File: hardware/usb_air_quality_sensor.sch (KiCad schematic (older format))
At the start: 21 parts

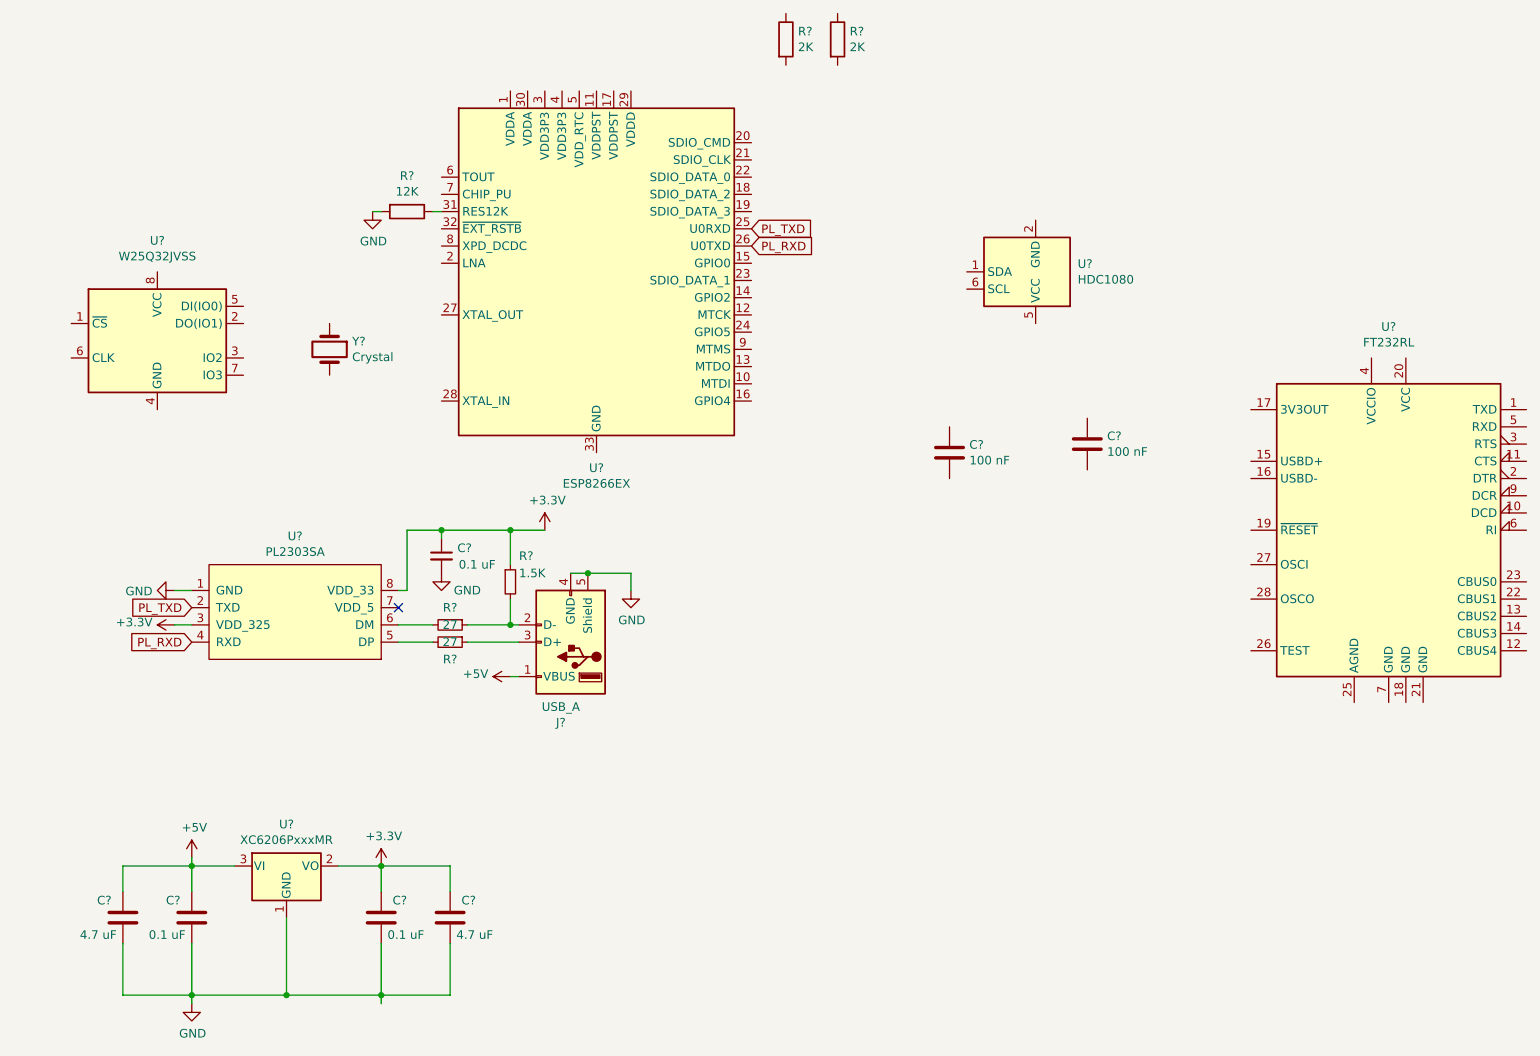
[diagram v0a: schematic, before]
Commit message: wip
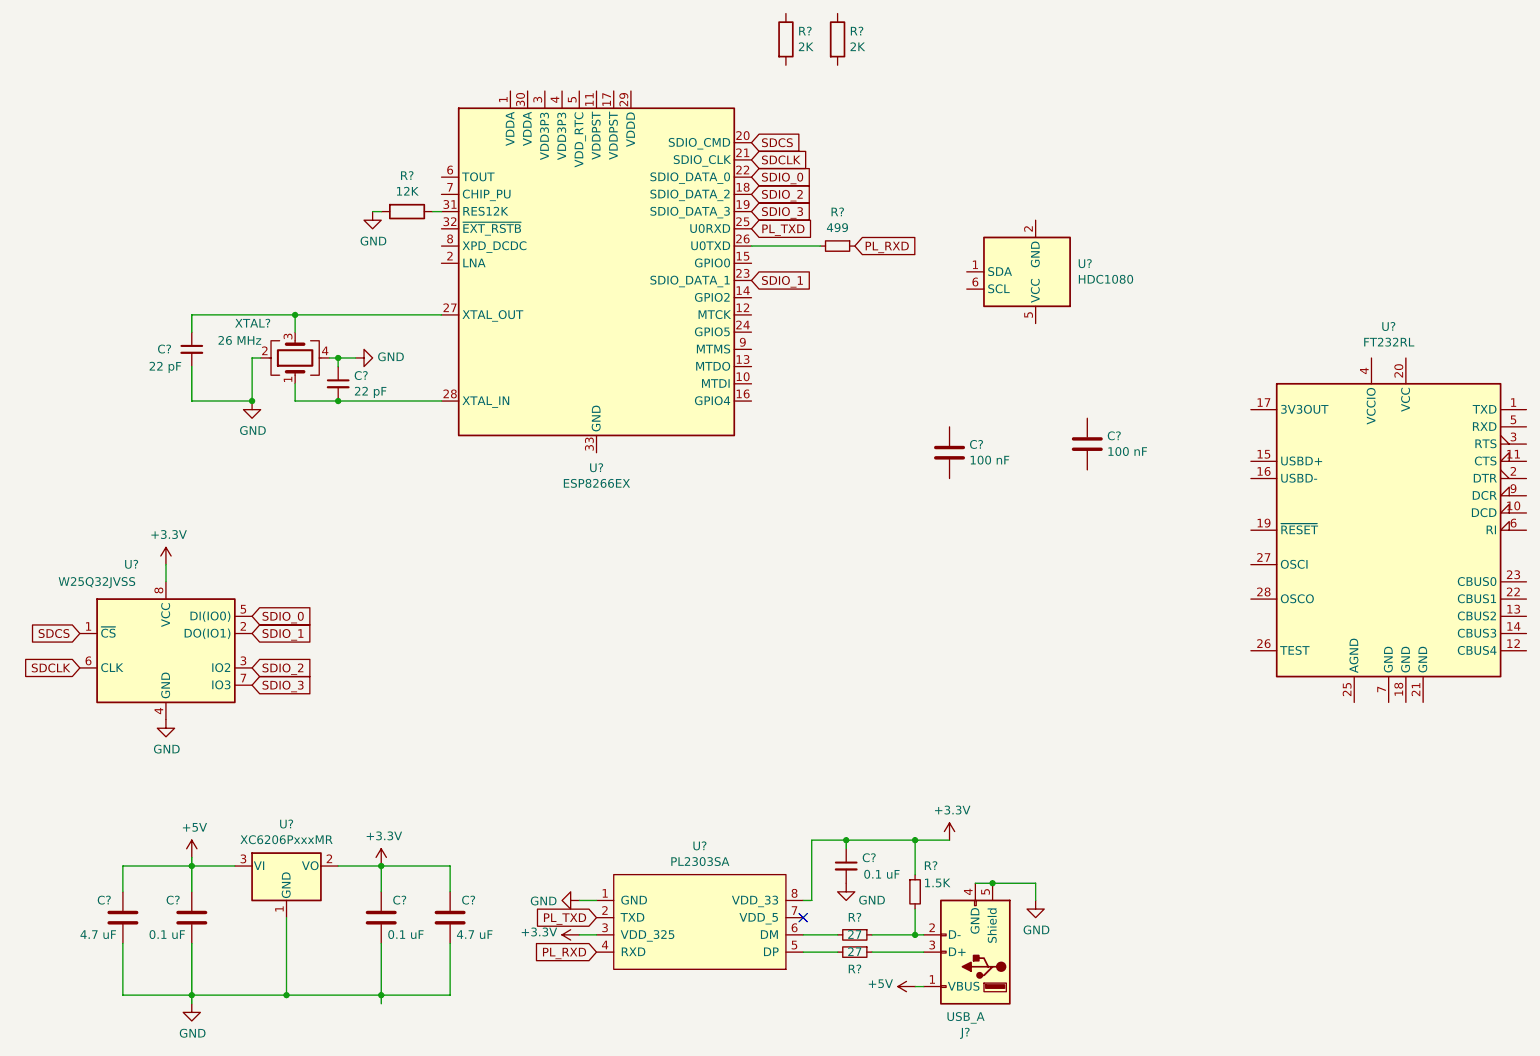
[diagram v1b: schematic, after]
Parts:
- removed Y?: Crystal, symbol Device:Crystal
- added C? (x2): 22 pF, symbol Device:C_Small
- added R?: 499, symbol Device:R_Small
- added XTAL?: 26 MHz, symbol Device:Crystal_GND24
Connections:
- net +3V3: now also U?.8 (VCC)
- net GND: now also U?.4 (GND), C?.1, C?.2, XTAL?.2, XTAL?.4
- net PL_RXD: now also R?.1; no longer U?.26 (U0TXD)
- net SDIO_2: now reaches U?.18 (SDIO_DATA_2)
- net SDIO_2: now also U?.3 (IO2)
- net SDIO_3: now reaches U?.19 (SDIO_DATA_3)
- net SDIO_3: now also U?.7 (IO3)
- net SDCS: now reaches U?.20 (SDIO_CMD)
- net SDCS: now also U?.1 (~CS)
- net SDCLK: now reaches U?.21 (SDIO_CLK)
- net SDCLK: now also U?.6 (CLK)
- net SDIO_0: now reaches U?.22 (SDIO_DATA_0)
- net SDIO_0: now also U?.5 (DI(IO0))
- net SDIO_1: now reaches U?.23 (SDIO_DATA_1)
- net SDIO_1: now also U?.2 (DO(IO1))
- net at U?.27 (XTAL_OUT): now also C?.1, XTAL?.3
- net at U?.28 (XTAL_IN): now also C?.2, XTAL?.1
- new net: R?.2, U?.26 (U0TXD)
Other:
- moved on the sheet: C?, J?, R?, U?
